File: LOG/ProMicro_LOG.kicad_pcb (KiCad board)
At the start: 2 copper layers, 17.8 x 30.5 mm, 16 parts, among them J1 Micro_SD_Card_Det, U1 DS3231MZ

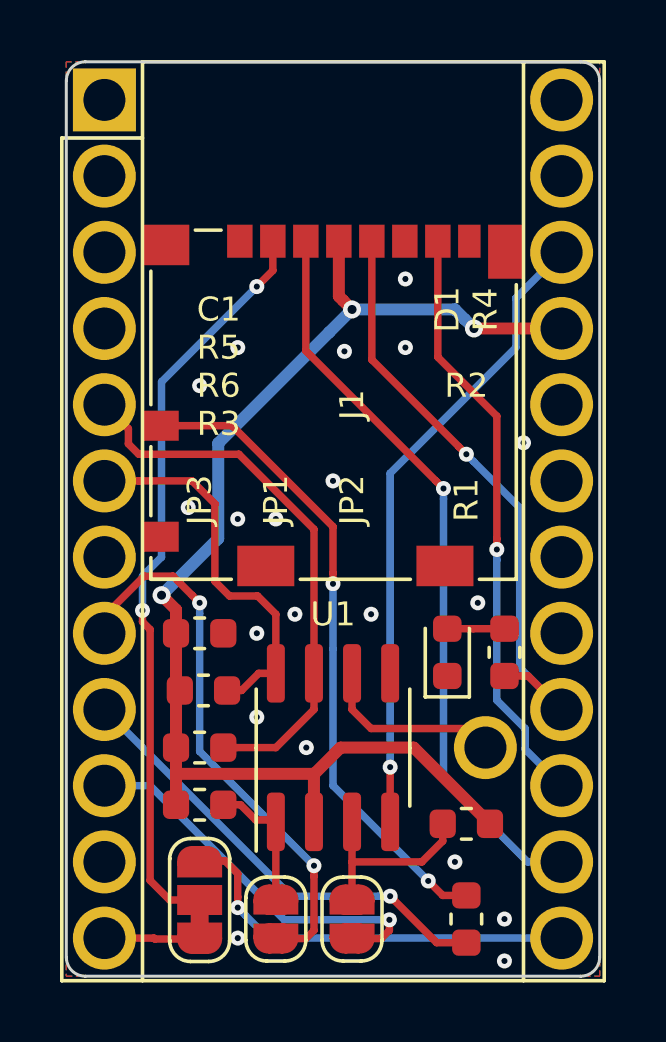
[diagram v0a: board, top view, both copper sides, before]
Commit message: update design
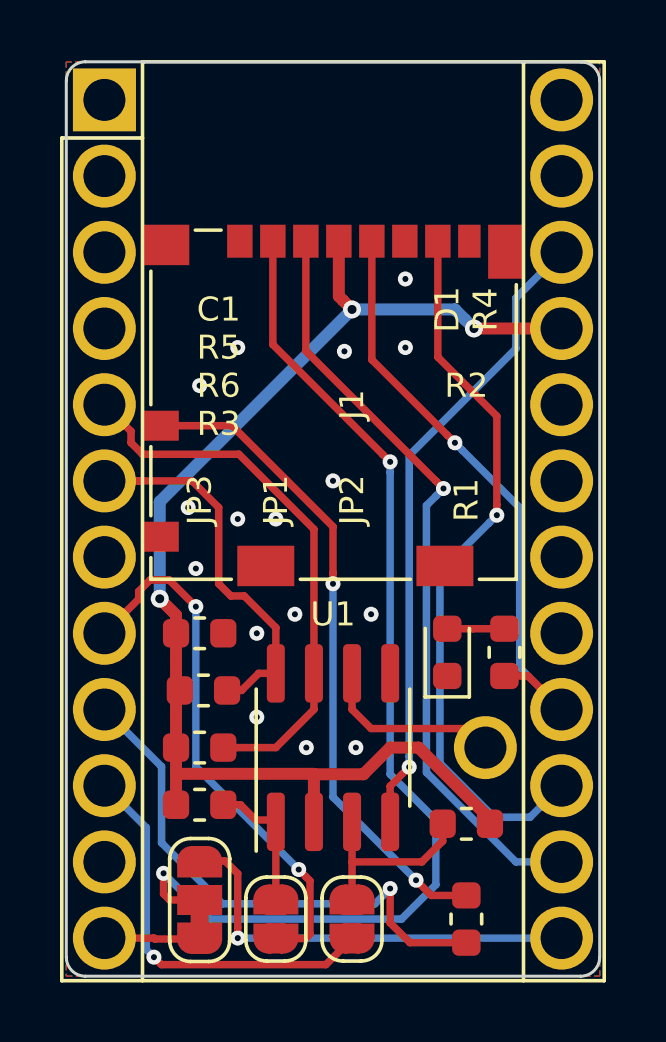
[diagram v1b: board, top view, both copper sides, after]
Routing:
- net CS: track 25.1 -> 35.9 mm
- net CIPO: track 19.9 -> 24.2 mm
- net BTN: track 15.3 -> 17.9 mm
- net COPI: track 24.9 -> 25.6 mm
- net CS0: track 13.8 -> 14.4 mm
- net PWM: track 18.6 -> 18.0 mm
- net GND: vias 20 -> 16
